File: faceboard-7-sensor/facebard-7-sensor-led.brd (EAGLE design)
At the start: 37 x 91.4 mm, 31 parts, among them Q1 QRE1113, Q2 QRE1113, Q3 QRE1113, Q4 QRE1113, Q5 QRE1113, Q6 QRE1113, Q7 QRE1113, U1 CD4051BE

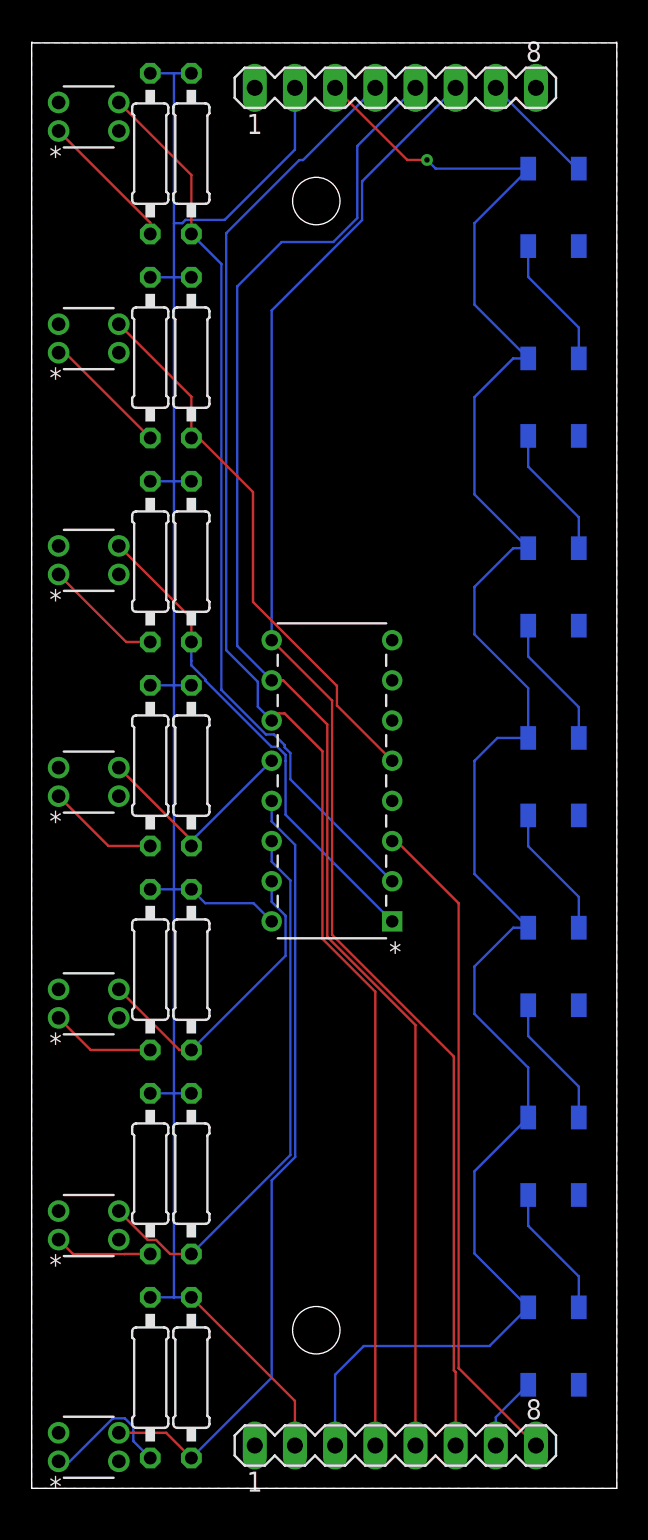
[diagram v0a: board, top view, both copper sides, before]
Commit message: routing
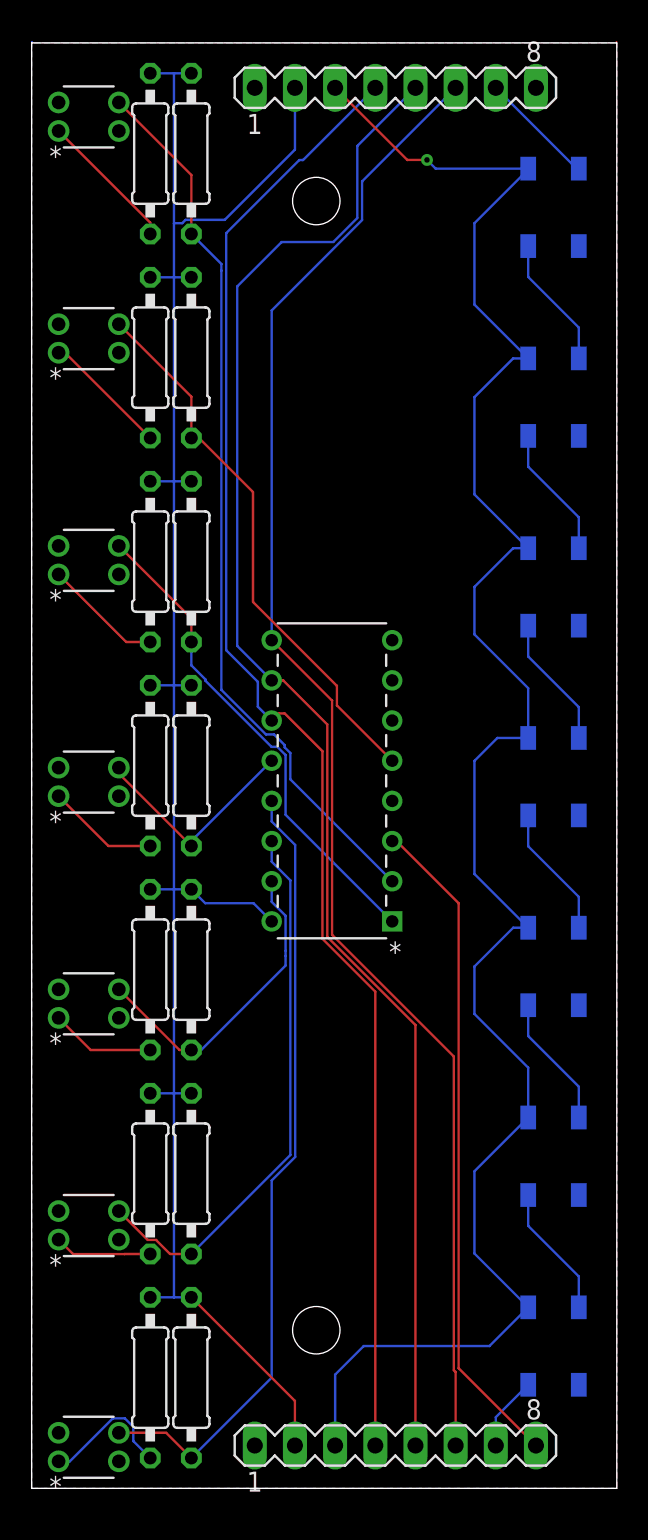
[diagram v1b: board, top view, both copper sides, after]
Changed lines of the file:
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@@
 <signal name="C0">
 <contactref element="U1" pad="13"/>
+<wire x1="15.18" y1="7" x2="15.18" y2="19.46894375" width="0.1524" layer="16"/>
+<wire x1="16.6659" y1="20.95484375" x2="15.18" y2="19.46894375" width="0.1524" layer="16"/>
+<wire x1="15.18" y1="43.47" x2="15.18" y2="42.16928125" width="0.1524" layer="16"/>
+<wire x1="15.18" y1="42.16928125" x2="16.6659" y2="40.68338125" width="0.1524" layer="16"/>
+<wire x1="16.6659" y1="40.68338125" x2="16.6659" y2="20.95484375" width="0.1524" layer="16"/>
 <contactref element="Q1" pad="3"/>
 <contactref element="R2" pad="1"/>
 <wire x1="5.515" y1="3.5134" x2="8.5066" y2="3.5134" width="0.1524" layer="1"/>
 <wire x1="8.5066" y1="3.5134" x2="10.1" y2="1.92" width="0.1524" layer="1"/>
-<wire x1="15.18" y1="7" x2="10.1" y2="1.92" width="0.1524" layer="16"/>
-<wire x1="15.18" y1="19.46894375" x2="15.18" y2="7" width="0.1524" layer="16"/>
-<wire x1="16.6659" y1="20.95484375" x2="15.18" y2="19.46894375" width="0.1524" layer="16"/>
-<wire x1="15.18" y1="43.47" x2="15.18" y2="42.16928125" width="0.1524" layer="16"/>
-<wire x1="15.18" y1="42.16928125" x2="16.6659" y2="40.68338125" width="0.1524" layer="16"/>
-<wire x1="16.6659" y1="40.68338125" x2="16.6659" y2="20.95484375" width="0.1524" layer="16"/>
+<wire x1="10.1" y1="1.92" x2="15.18" y2="7" width="0.1524" layer="16"/>
 </signal>
 <signal name="GND">
@@
 </signal>
 <signal name="C1">
+<contactref element="U1" pad="14"/>
+<wire x1="15.18" y1="40.93" x2="15.18" y2="39.62928125" width="0.1524" layer="16"/>
+<wire x1="15.18" y1="39.62928125" x2="16.3611" y2="38.44818125" width="0.1524" layer="16"/>
+<wire x1="16.3611" y1="21.0811" x2="16.3611" y2="38.44818125" width="0.1524" layer="16"/>
 <contactref element="Q2" pad="3"/>
 <contactref element="R4" pad="1"/>
-<contactref element="U1" pad="14"/>
 <wire x1="5.515" y1="17.5334" x2="7.3394" y2="15.709" width="0.1524" layer="1"/>
 <wire x1="7.3394" y1="15.709" x2="7.8682375" y2="15.709" width="0.1524" layer="1"/>
 <wire x1="8.7572375" y1="14.82" x2="10.1" y2="14.82" width="0.1524" layer="1"/>
 <wire x1="7.8682375" y1="15.709" x2="8.7572375" y2="14.82" width="0.1524" layer="1"/>
-<wire x1="15.18" y1="40.93" x2="15.18" y2="39.62928125" width="0.1524" layer="16"/>
-<wire x1="15.18" y1="39.62928125" x2="16.3611" y2="38.44818125" width="0.1524" layer="16"/>
-<wire x1="16.3611" y1="38.44818125" x2="16.3611" y2="21.0811" width="0.1524" layer="16"/>
-<wire x1="16.3611" y1="21.0811" x2="10.1" y2="14.82" width="0.1524" layer="16"/>
+<wire x1="10.1" y1="14.82" x2="16.3611" y2="21.0811" width="0.1524" layer="16"/>
 </signal>
 <signal name="N$5">
@@
 </signal>
 <signal name="C2">
+<contactref element="U1" pad="15"/>
+<wire x1="15.18" y1="38.39" x2="15.18" y2="37.08928125" width="0.1524" layer="16"/>
+<wire x1="15.18" y1="37.08928125" x2="16.0563" y2="36.21298125" width="0.1524" layer="16"/>
+<wire x1="16.0563" y1="36.21298125" x2="16.0563" y2="34" width="0.1524" layer="16"/>
 <contactref element="Q3" pad="3"/>
 <contactref element="R6" pad="1"/>
-<contactref element="U1" pad="15"/>
+<wire x1="16.0563" y1="34" x2="16.0563" y2="33.6763" width="0.1524" layer="16"/>
 <wire x1="5.515" y1="31.5534" x2="9.3484" y2="27.72" width="0.1524" layer="1"/>
 <wire x1="9.3484" y1="27.72" x2="10.1" y2="27.72" width="0.1524" layer="1"/>
-<wire x1="15.18" y1="38.39" x2="15.18" y2="37.08928125" width="0.1524" layer="16"/>
-<wire x1="15.18" y1="37.08928125" x2="16.0563" y2="36.21298125" width="0.1524" layer="16"/>
-<wire x1="16.0563" y1="36.21298125" x2="16.0563" y2="33.6763" width="0.1524" layer="16"/>
-<wire x1="16.0563" y1="33.6763" x2="10.1" y2="27.72" width="0.1524" layer="16"/>
+<wire x1="16.0563" y1="33.6763" x2="16.0563" y2="33.0563" width="0.1524" layer="16"/>
+<wire x1="10.72" y1="27.72" x2="10.1" y2="27.72" width="0.1524" layer="16"/>
+<wire x1="16.0563" y1="33.0563" x2="10.72" y2="27.72" width="0.1524" layer="16"/>
 </signal>
 <signal name="N$7">
@@
 </signal>
 <signal name="C3">
+<contactref element="U1" pad="12"/>
 <contactref element="Q4" pad="3"/>
 <contactref element="R8" pad="1"/>
-<contactref element="U1" pad="12"/>
-<wire x1="5.515" y1="45.5734" x2="10.1" y2="40.9884" width="0.1524" layer="1"/>
-<wire x1="10.1" y1="40.9884" x2="10.1" y2="40.62" width="0.1524" layer="1"/>
 <wire x1="15.18" y1="46.01" x2="10.1" y2="40.93" width="0.1524" layer="16"/>
 <wire x1="10.1" y1="40.93" x2="10.1" y2="40.62" width="0.1524" layer="16"/>
+<wire x1="10.1" y1="40.62" x2="5.515" y2="45.205" width="0.1524" layer="1"/>
+<wire x1="5.515" y1="45.205" x2="5.515" y2="45.5734" width="0.1524" layer="1"/>
 </signal>
 <signal name="N$9">
@@
 <contactref element="Q5" pad="3"/>
 <contactref element="R10" pad="1"/>
-<contactref element="U1" pad="1"/>
 <wire x1="5.515" y1="59.5934" x2="10.1" y2="55.0084" width="0.1524" layer="1"/>
 <wire x1="10.1" y1="55.0084" x2="10.1" y2="53.52" width="0.1524" layer="1"/>
-<wire x1="22.8" y1="35.85" x2="16.0563" y2="42.5937" width="0.1524" layer="16"/>
-<wire x1="10.1" y1="52.32928125" x2="10.1" y2="53" width="0.1524" layer="16"/>
-<wire x1="10.1" y1="53" x2="10.1" y2="53.52" width="0.1524" layer="16"/>
-<wire x1="16.0563" y1="42.5937" x2="16.0563" y2="46" width="0.1524" layer="16"/>
-<wire x1="16.0563" y1="46" x2="16.0563" y2="46.37298125" width="0.1524" layer="16"/>
+<wire x1="10.1" y1="52.0372375" x2="10.1" y2="53.52" width="0.1524" layer="16"/>
+<wire x1="16.0563" y1="42.5937" x2="16.0563" y2="46.37298125" width="0.1524" layer="16"/>
 <wire x1="16.0563" y1="46.37298125" x2="15.54298125" y2="46.8863" width="0.1524" layer="16"/>
 <wire x1="15.54298125" y1="46.8863" x2="15.1733625" y2="46.8863" width="0.1524" layer="16"/>
 <wire x1="15.1733625" y1="46.8863" x2="10.989" y2="51.0706625" width="0.1524" layer="16"/>
 <wire x1="10.989" y1="51.0706625" x2="10.989" y2="51.1482375" width="0.1524" layer="16"/>
-<wire x1="10.1" y1="52.0372375" x2="10.1" y2="52.32928125" width="0.1524" layer="16"/>
 <wire x1="10.989" y1="51.1482375" x2="10.1" y2="52.0372375" width="0.1524" layer="16"/>
+<contactref element="U1" pad="1"/>
+<wire x1="22.8" y1="35.85" x2="16.0563" y2="42.5937" width="0.1524" layer="16"/>
 </signal>
 <signal name="N$11">
@@
 <contactref element="Q6" pad="3"/>
 <contactref element="R12" pad="1"/>
-<contactref element="U1" pad="5"/>
 <wire x1="5.515" y1="73.6134" x2="10.1" y2="69.0284" width="0.1524" layer="1"/>
 <wire x1="10.1" y1="69.0284" x2="10.1" y2="66.42" width="0.1524" layer="1"/>
-<wire x1="22.8" y1="46.01" x2="19.3048" y2="49.5052" width="0.1524" layer="1"/>
 <wire x1="14" y1="56.04928125" x2="14" y2="63" width="0.1524" layer="1"/>
 <wire x1="19.3048" y1="49.5052" x2="19.3048" y2="50.74448125" width="0.1524" layer="1"/>
@@
 <wire x1="14" y1="63" x2="10.58" y2="66.42" width="0.1524" layer="1"/>
 <wire x1="10.58" y1="66.42" x2="10.1" y2="66.42" width="0.1524" layer="1"/>
+<contactref element="U1" pad="5"/>
+<wire x1="22.8" y1="46.01" x2="19.3048" y2="49.5052" width="0.1524" layer="1"/>
 </signal>
 <signal name="N$13">
@@
 </signal>
 <signal name="C6">
-<contactref element="Q7" pad="3"/>
-<contactref element="R14" pad="1"/>
 <contactref element="U1" pad="2"/>
-<wire x1="5.515" y1="87.6334" x2="10.1" y2="83.0484" width="0.1524" layer="1"/>
-<wire x1="10.1" y1="83.0484" x2="10.1" y2="79.32" width="0.1524" layer="1"/>
 <wire x1="22.8" y1="38.39" x2="16.3611" y2="44.8289" width="0.1524" layer="16"/>
 <wire x1="16.3611" y1="44.8289" x2="16.3611" y2="46.4992375" width="0.1524" layer="16"/>
 <wire x1="16" y1="46.8603375" x2="16" y2="47" width="0.1524" layer="16"/>
 <wire x1="16.3611" y1="46.4992375" x2="16" y2="46.8603375" width="0.1524" layer="16"/>
-<wire x1="11.9989" y1="77.4211" x2="10.1" y2="79.32" width="0.1524" layer="16"/>
 <wire x1="16" y1="47" x2="15.3263" y2="47.6737" width="0.1524" layer="16"/>
 <wire x1="15.3263" y1="47.6737" x2="14.81701875" y2="47.6737" width="0.1524" layer="16"/>
 <wire x1="14.81701875" y1="47.6737" x2="11.9989" y2="50.49181875" width="0.1524" layer="16"/>
-<wire x1="11.9989" y1="50.49181875" x2="11.9989" y2="77.4211" width="0.1524" layer="16"/>
+<wire x1="11.9989" y1="50.49181875" x2="11.9989" y2="77" width="0.1524" layer="16"/>
+<contactref element="Q7" pad="3"/>
+<contactref element="R14" pad="1"/>
+<wire x1="5.515" y1="87.6334" x2="10.1" y2="83.0484" width="0.1524" layer="1"/>
+<wire x1="10.1" y1="83.0484" x2="10.1" y2="79.32" width="0.1524" layer="1"/>
+<wire x1="11.9989" y1="77" x2="11.9989" y2="77.4211" width="0.1524" layer="16"/>
+<wire x1="11.9989" y1="77.4211" x2="10.1" y2="79.32" width="0.1524" layer="16"/>
 </signal>
 <signal name="SIG">
